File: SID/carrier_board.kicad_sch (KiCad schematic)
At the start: 0 parts

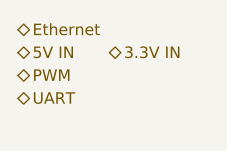
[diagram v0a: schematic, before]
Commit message: Feat(SID): basically complete
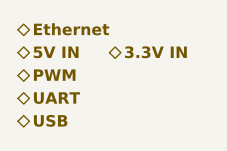
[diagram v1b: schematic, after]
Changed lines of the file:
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@@
-(kicad_sch (version 20230819) (generator eeschema)
-  (paper "A4")
-  (hierarchical_label "PWM" (shape bidirectional) (at 109.22 91.44 0) (fields_autoplaced)
-    (effects (font (size 1.27 1.27)) (justify left))
-  )
-  (hierarchical_label "5V IN" (shape bidirectional) (at 109.22 88.9 0) (fields_autoplaced)
-    (effects (font (size 1.27 1.27)) (justify left))
-  )
-  (hierarchical_label "Ethernet" (shape bidirectional) (at 109.22 86.36 0) (fields_autoplaced)
-    (effects (font (size 1.27 1.27)) (justify left))
-  )
-  (hierarchical_label "3.3V IN" (shape bidirectional) (at 119.38 88.9 0) (fields_autoplaced)
-    (effects (font (size 1.27 1.27)) (justify left))
-  )
-  (hierarchical_label "UART" (shape bidirectional) (at 109.22 93.98 0) (fields_autoplaced)
-    (effects (font (size 1.27 1.27)) (justify left))
-  )
+(kicad_sch
+	(version 20240101)
+	(generator "eeschema")
+	(generator_version "8.99")
+	(paper "A4")
+	(hierarchical_label "PWM"
+		(shape bidirectional)
+		(at 109.22 91.44 0)
+		(fields_autoplaced yes)
+		(effects
+			(font
+				(face "JetBrains Mono")
+				(size 1.27 1.27)
+				(thickness 0.254)
+				(bold yes)
+			)
+			(justify left)
+		)
+	)
+	(hierarchical_label "5V IN"
+		(shape bidirectional)
+		(at 109.22 88.9 0)
+		(fields_autoplaced yes)
+		(effects
+			(font
+				(face "JetBrains Mono")
+				(size 1.27 1.27)
+				(thickness 0.254)
+				(bold yes)
+			)
+			(justify left)
+		)
+	)
+	(hierarchical_label "Ethernet"
+		(shape bidirectional)
+		(at 109.22 86.36 0)
+		(fields_autoplaced yes)
+		(effects
+			(font
+				(face "JetBrains Mono")
+				(size 1.27 1.27)
+				(thickness 0.254)
+				(bold yes)
+			)
+			(justify left)
+		)
+	)
+	(hierarchical_label "3.3V IN"
+		(shape bidirectional)
+		(at 119.38 88.9 0)
+		(fields_autoplaced yes)
+		(effects
+			(font
+				(face "JetBrains Mono")
+				(size 1.27 1.27)
+				(thickness 0.254)
+				(bold yes)
+			)
+			(justify left)
+		)
+	)
+	(hierarchical_label "UART"
+		(shape bidirectional)
+		(at 109.22 93.98 0)
+		(fields_autoplaced yes)
+		(effects
+			(font
+				(face "JetBrains Mono")
+				(size 1.27 1.27)
+				(thickness 0.254)
+				(bold yes)
+			)
+			(justify left)
+		)
+	)
+	(hierarchical_label "USB"
+		(shape bidirectional)
+		(at 109.22 96.52 0)
+		(fields_autoplaced yes)
+		(effects
+			(font
+				(face "JetBrains Mono")
+				(size 1.27 1.27)
+				(thickness 0.254)
+				(bold yes)
+			)
+			(justify left)
+		)
+	)
 )
